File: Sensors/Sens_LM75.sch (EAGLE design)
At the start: 13 parts, among them IC2 SI7005, X1 SCL, X2 3v3, X3 GND, X4 SCL, X5 SDA, X6 SDA, X7 3v3, X8 GND

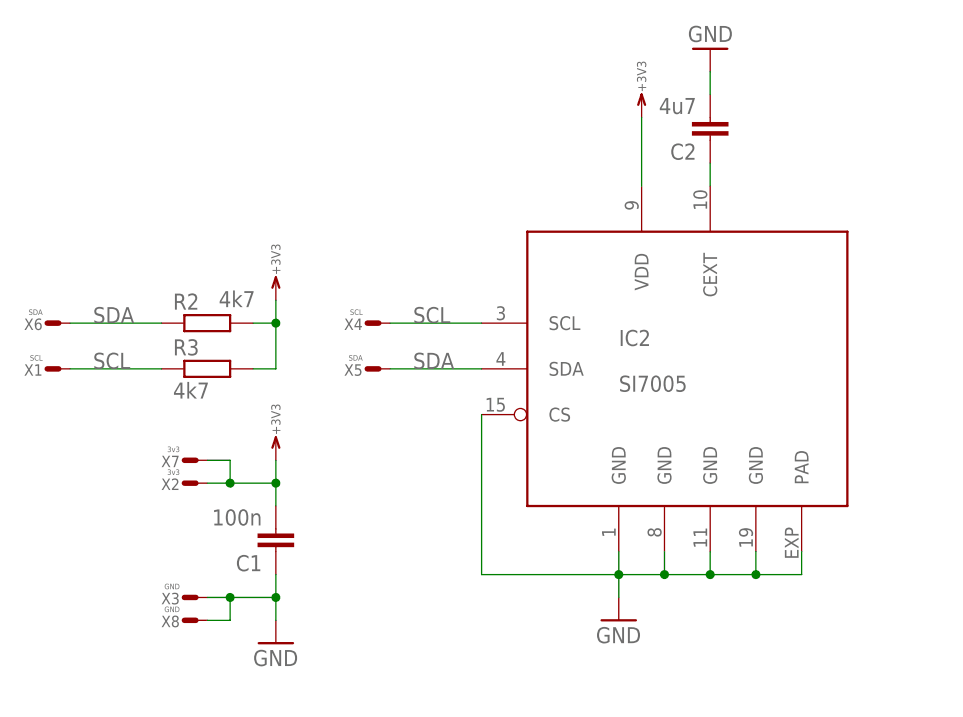
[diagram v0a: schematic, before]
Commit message: Typo correction and more elegance presentation
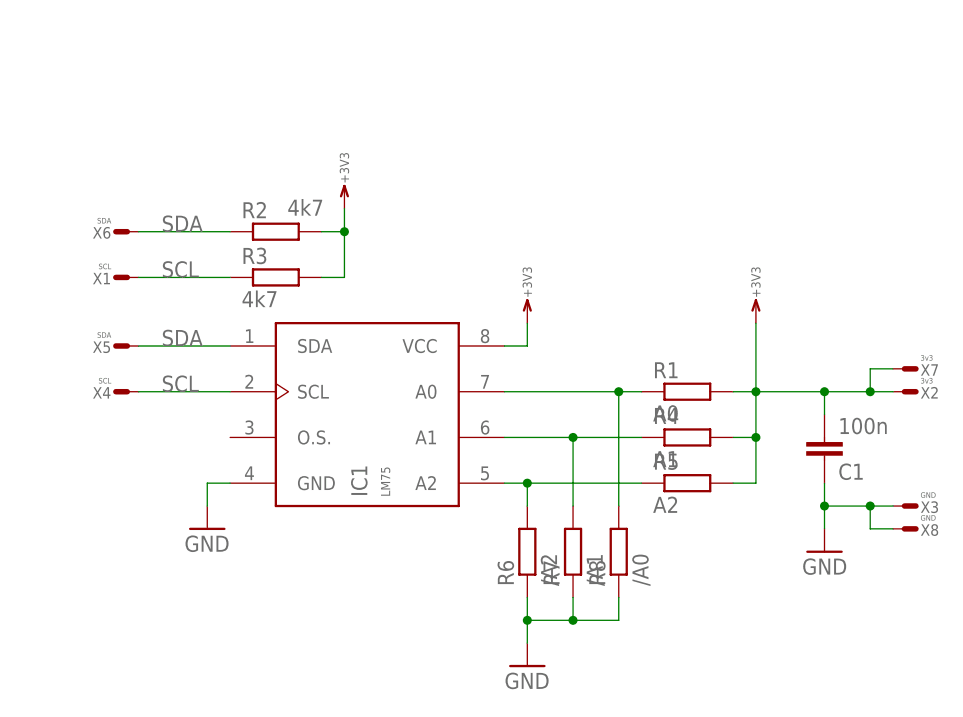
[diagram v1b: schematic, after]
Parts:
- removed C2: 4u7, RCL:C0603
- removed IC2: SI7005, Sensors:SI7005
- added IC1: LM75, Sensors:LM75M
- added R1: A0, RCL:R0603
- added R4: A1, RCL:R0603
- added R5: A2, RCL:R0603
- added R6: /A2, RCL:R0603
- added R7: /A1, RCL:R0603
- added R8: /A0, RCL:R0603
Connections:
- new net N$2: IC1.A1, R4.1, R7.2
- new net N$3: IC1.A2, R5.1, R6.2
- net +3V3: now also IC1.VCC, R1.2, R4.2, R5.2; no longer IC2.VDD
- net GND: now also IC1.GND, R6.1, R7.1, R8.1; no longer C2.2, IC2.CS, IC2.GND@1, IC2.GND@11, IC2.GND@19, IC2.GND@8, IC2.PAD
- net N$1: now also IC1.A0, R1.1, R8.2; no longer C2.1, IC2.CEXT
- net SCL: now also IC1.SCL; no longer IC2.SCL
- net SDA: now also IC1.SDA; no longer IC2.SDA
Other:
- moved on the sheet: C1, R2, R3, X1, X2, X3, X4, X5, X6, X7, X8
